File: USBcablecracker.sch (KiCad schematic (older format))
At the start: 52 parts, among them P1 USB_A, P10 USB_A, P11 USB_B, P12 CONN_01X09, P2 CONN_01X02, P3 USB_B-Micro, P6 CONN_01X09, P7 USB_B-Mini, P8 USB_B-Micro-3.0, P9 USB_TYPEC-S, SW1 Switch_SPDT_x2, U1 ATmega32U4-AU, U2 LMV358, U3 AD623, Y1 16MHz

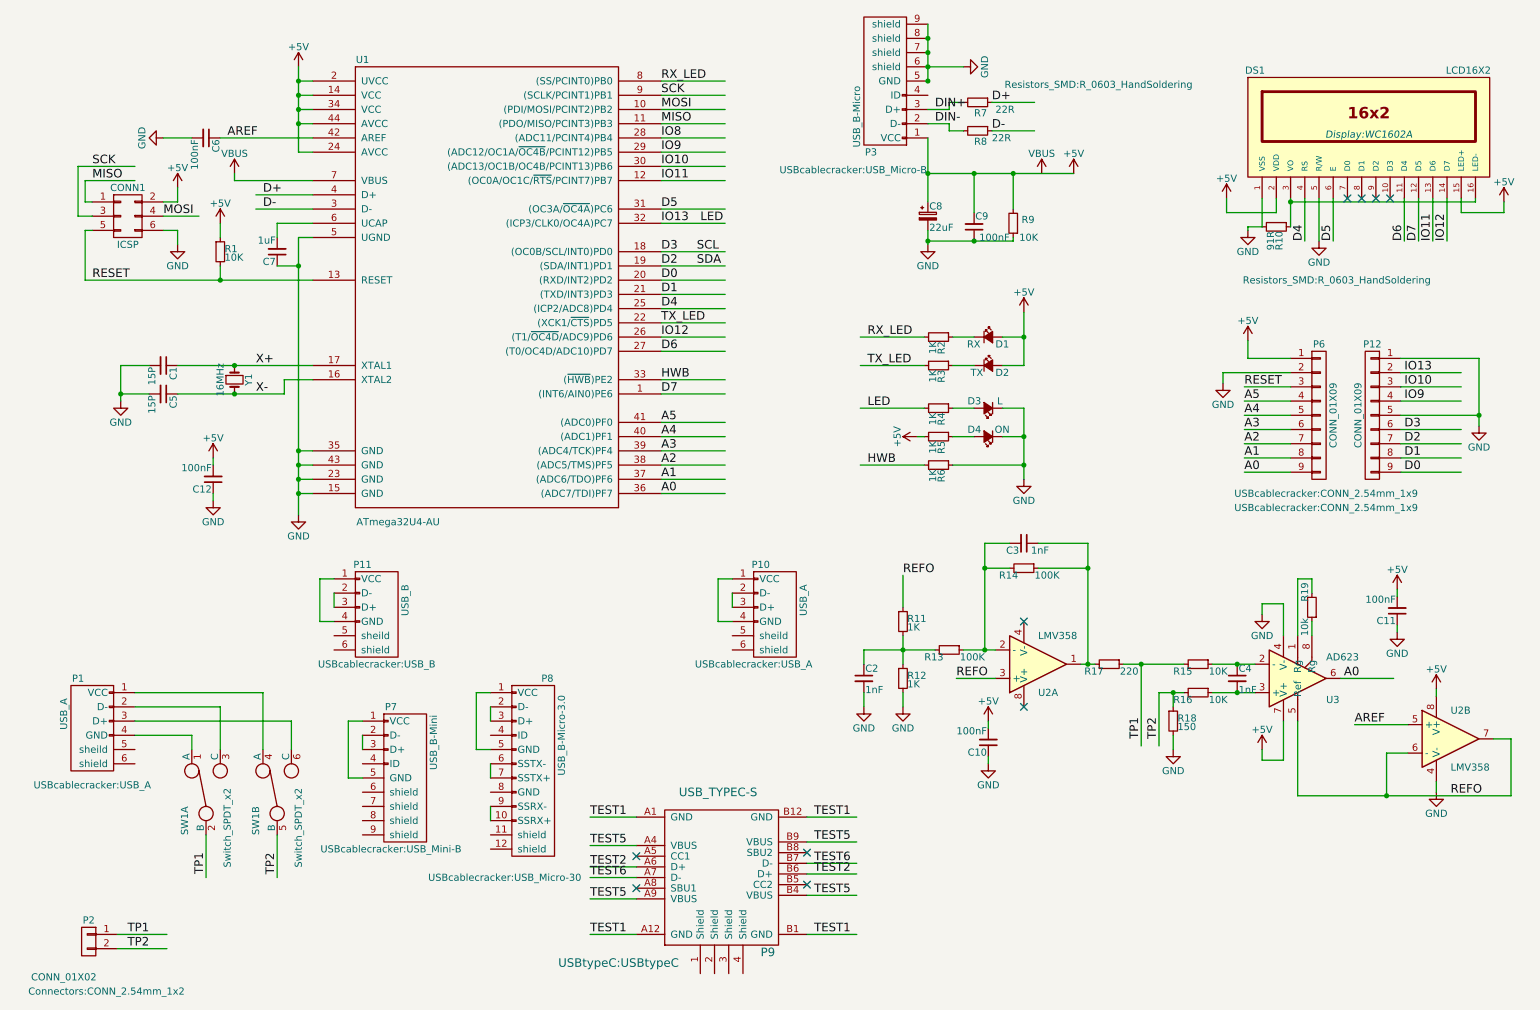
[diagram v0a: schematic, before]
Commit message: update
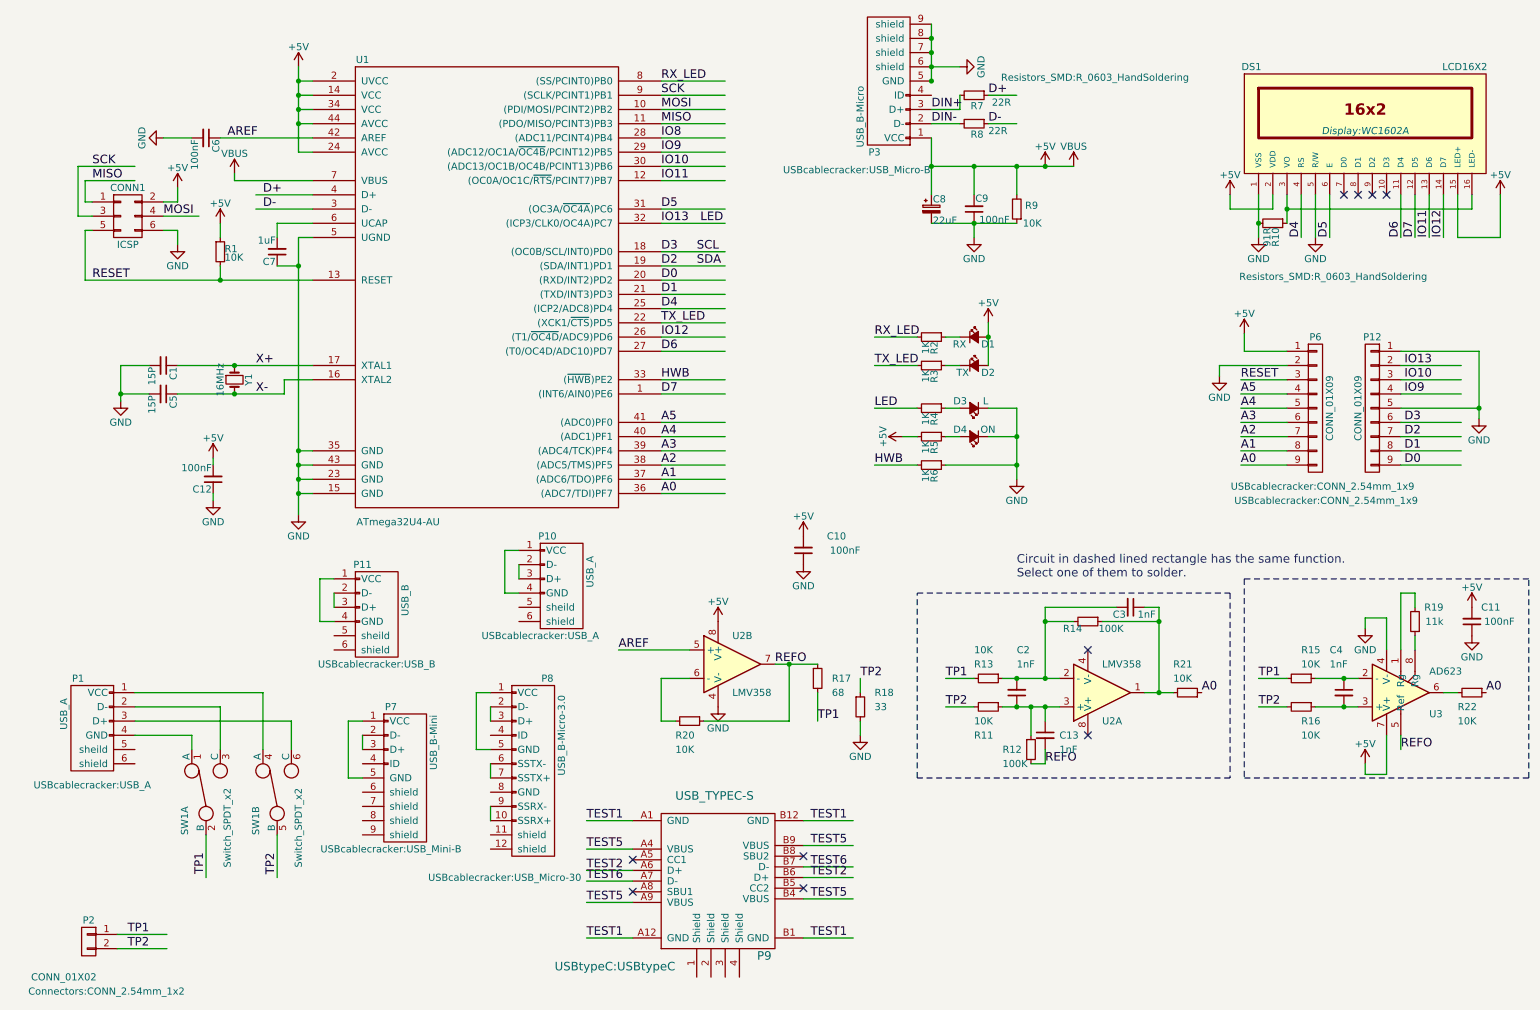
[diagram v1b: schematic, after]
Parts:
- added C13: 1nF, Capacitors_SMD:C_0603_HandSoldering, symbol C_Small
- added R20, R21, R22: 10K, Resistors_SMD:R_0603_HandSoldering, symbol R_Small
- R11: value 1K -> 10K
- R12: value 1K -> 100K
- R13: value 100K -> 10K
- R17: value 220 -> 68
- R18: value 150 -> 33
- R19: value 10k -> 11k
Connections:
- wire segments 234 -> 220
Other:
- note added: "Circuit in dashed lined rectangle has the same function.\nSelect one of them to solder."
- moved on the sheet: C10, C11, C2, C3, C4, C8, C9, D1, D2, D3, D4, DS1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
